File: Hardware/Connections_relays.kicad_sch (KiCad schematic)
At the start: 51 parts, among them J2 Conn_01x02, J3 1040310811, J4 Conn_01x02, J6 Conn_01x02, J7 Conn_01x02, Q11 IRLML0030, Q6 IRLML0030, Q8 IRLML0030, Q9 IRLML0030, U11 W25Q128JVS

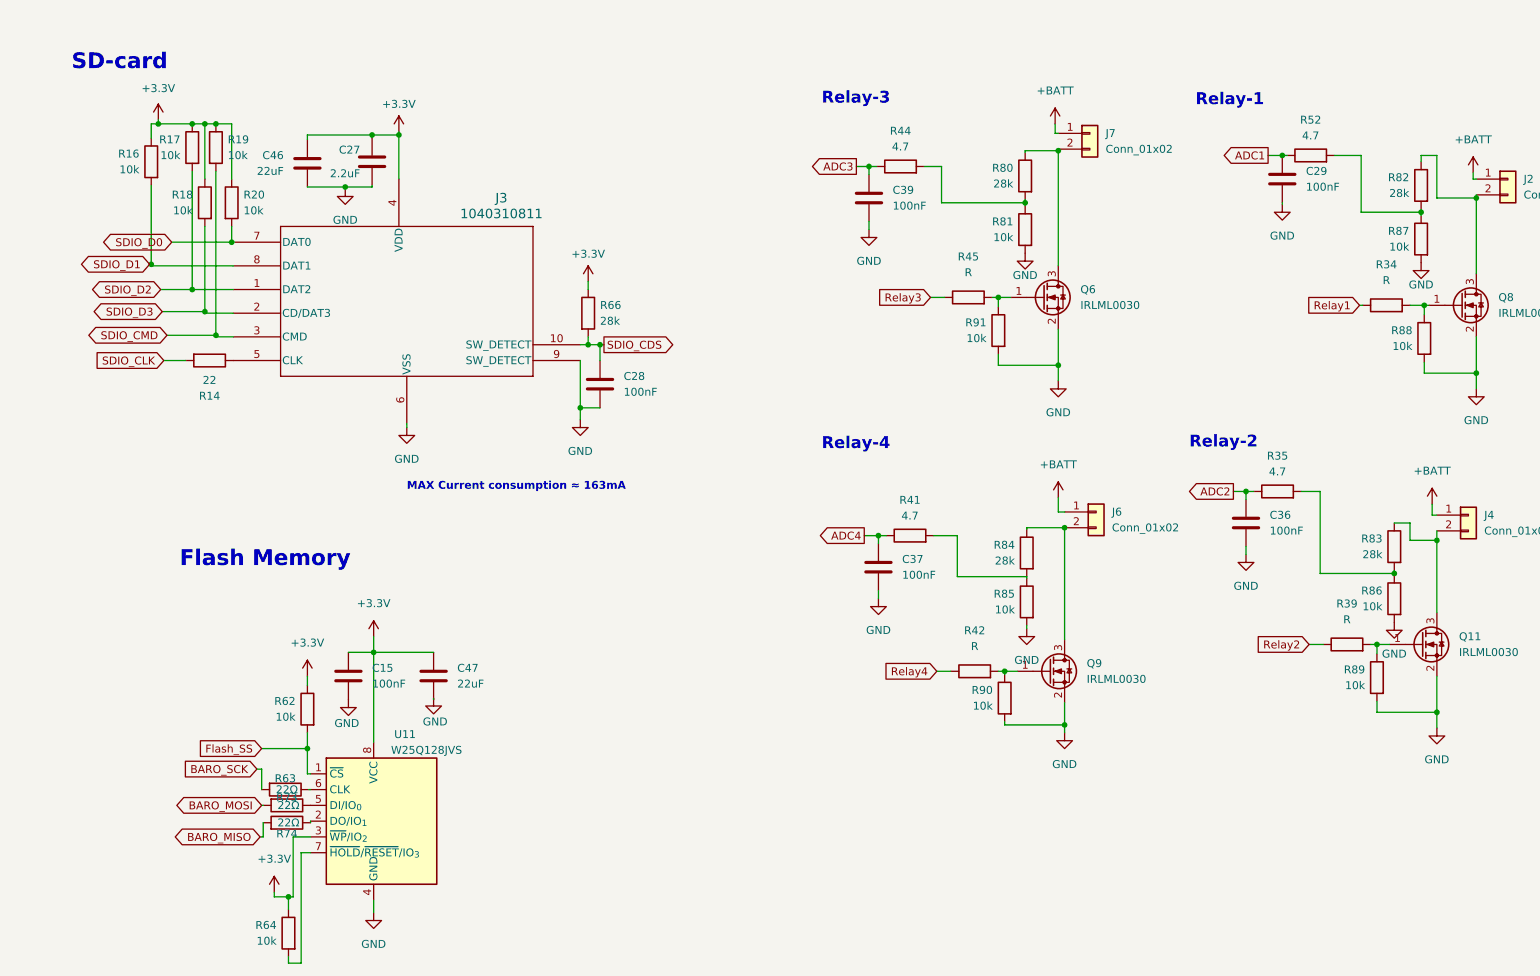
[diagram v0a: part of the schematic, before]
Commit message: Changed footprints, generated BOM
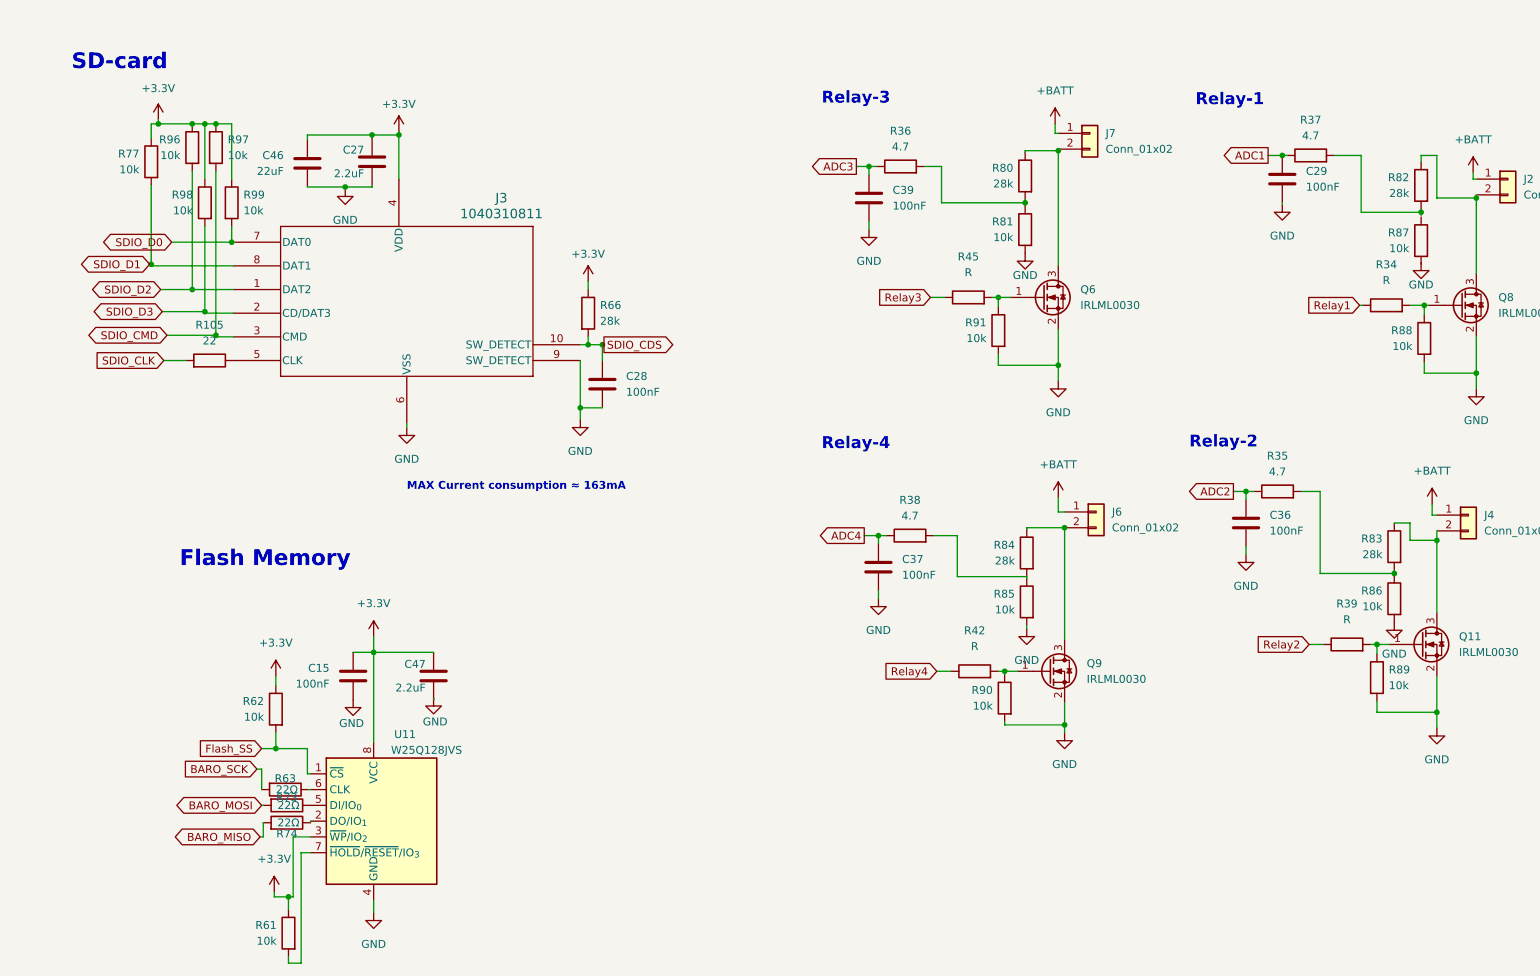
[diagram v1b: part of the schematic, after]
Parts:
- removed R14: 22, Resistor_SMD:R_0402_1005Metric, symbol Device:R
- removed R16, R17, R18, R19, R20, R64: 10k, Resistor_SMD:R_0402_1005Metric, symbol Device:R
- removed R41, R44, R52: 4.7, Resistor_SMD:R_0402_1005Metric, symbol Device:R
- added R105: 22, Resistor_SMD:R_0603_1608Metric, symbol Device:R
- added R36, R37, R38: 4.7, Resistor_SMD:R_0603_1608Metric, symbol Device:R
- added R61, R77, R96, R97, R98, R99: 10k, Resistor_SMD:R_0603_1608Metric, symbol Device:R
- C15, C28, C29, C36, C37, C39: footprint Capacitor_SMD:C_0402_1005Metric -> Capacitor_SMD:C_0603_1608Metric; Distributer Link https://www.ozdisan.com/p/smt-smd-ve-mlcc-kapasitorler-184/murata-grt155r71e104ke01d-1074547 -> https://www.ozdisan.com/p/smt-smd-ve-mlcc-kapasitorler-184/samsung-cl10b104ko8wpnc-522227; Part Number GRT155R71E104KE01D -> CL10B104KO8WPNC
- C27: footprint Capacitor_SMD:C_0402_1005Metric -> Capacitor_SMD:C_0603_1608Metric; Distributer Link http://ozdisan.com/p/smt-smd-ve-mlcc-kapasitorler-184/murat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 -> https://www.ozdisan.com/p/smt-smd-ve-mlcc-kapasitorler-184/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; Part Number GRT155C81A225ME13D -> CL10B225KP8NNNC
- C47: value 22uF -> 2.2uF; footprint Capacitor_SMD:C_0805_2012Metric -> Capacitor_SMD:C_0603_1608Metric; Distributer Link https://www.ozdisan.com/p/smt-smd-ve-mlcc-kapasitorler-184/samsung-cl21a226koqnnne-399002 -> https://www.ozdisan.com/p/smt-smd-ve-mlcc-kapasitorler-184/samsung-cl10b225kp8nnnc-359581; Part Number CL21A226KOQNNNE -> CL10B225KP8NNNC
- J2, J4, J6, J7: now left out of the parts list
- R35: footprint Resistor_SMD:R_0402_1005Metric -> Resistor_SMD:R_0603_1608Metric; Distributer Link https://www.ozdisan.com/p/smt-smd-ve-cip-direncler-194/royalohm-cq02wgj047jtce-587859 -> https://www.ozdisan.com/p/smt-smd-ve-cip-direncler-194/royalohm-cq03saf470kt5e-587940; Part Number CQ02WGJ047JTCE -> CQ03SAF470KT5E
- R62, R88, R89, R90, R91: footprint Resistor_SMD:R_0402_1005Metric -> Resistor_SMD:R_0603_1608Metric; Distributer Link https://www.ozdisan.com/p/smt-smd-ve-cip-direncler-194/roya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 -> https://www.ozdisan.com/p/smt-smd-ve-cip-direncler-194/viki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; Part Number CQ02WGF1002TCE -> CRT03J7E1002
- R81, R85, R86, R87: footprint Resistor_SMD:R_0402_1005Metric -> Resistor_SMD:R_0603_1608Metric; Distributer Link https://www.ozdisan.com/p/smt-smd-ve-cip-direncler-194/royalohm-cq02wgf1002tce-587902 -> https://www.ozdisan.com/p/smt-smd-ve-cip-direncler-194/royalohm-tc0350b1002t5f-700101; Part Number CQ02WGF1002TCE -> TC0350B1002T5F
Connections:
- net +3.3V: now also R61.1, R77.1, R96.1, R97.1, R98.1, R99.1
- net ADC1: now also R37.1
- net ADC3: now also R36.1
- net ADC4: now also R38.1
- net GND: no longer R87.2
- net SDIO_CLK: now also R105.2
- net SDIO_CMD: now also R97.2
- net SDIO_D0: now also R99.2
- net SDIO_D1: now also R77.2
- net SDIO_D2: now also R96.2
- net SDIO_D3: now also R98.2
- net at R80.2, R81.1: now also R36.2
- net at R82.2: now also R37.2; no longer R87.1
- net at J3.5 (CLK): now also R105.1
- net at R84.2, R85.1: now also R38.2
- net at U11.7 (~{HOLD}/~{RESET}/IO_{3}): now also R61.2

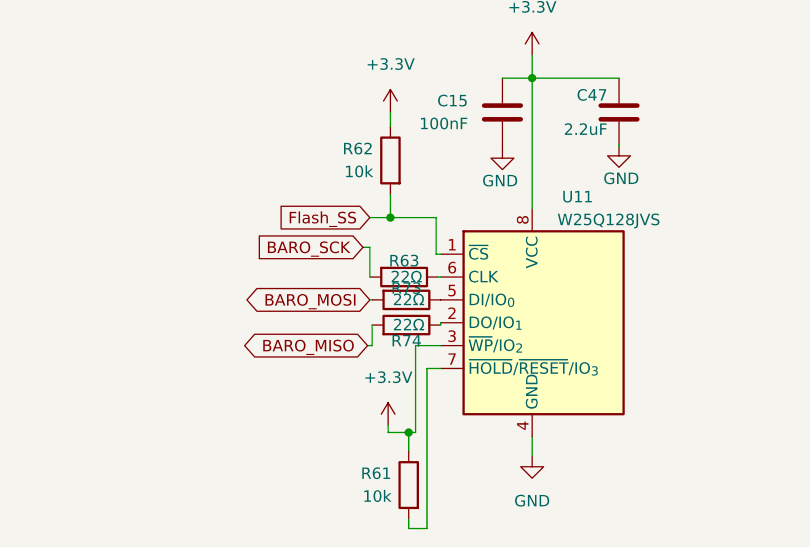
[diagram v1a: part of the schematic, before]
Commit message: Final changes
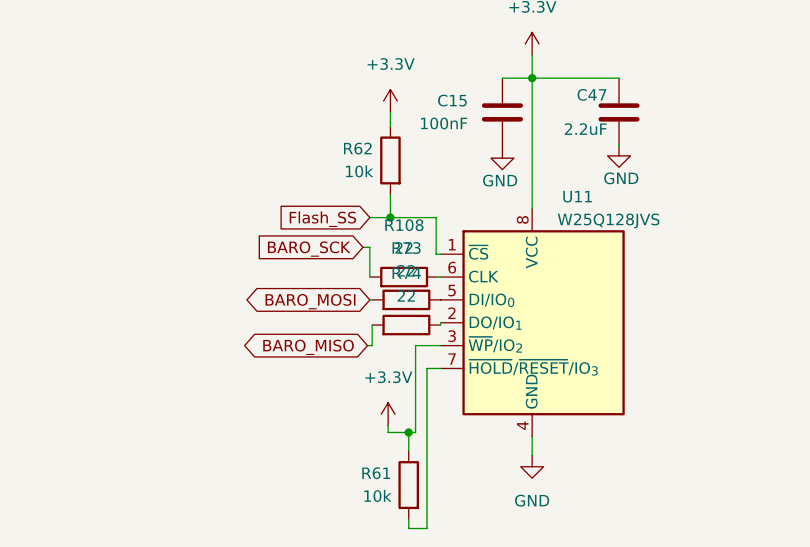
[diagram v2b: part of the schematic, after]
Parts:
- removed R63: 22Ω, Resistor_SMD:R_0402_1005Metric, symbol Device:R
- added R108: 22, Resistor_SMD:R_0603_1608Metric, symbol Device:R
- R73, R74: value 22Ω -> 22; footprint Resistor_SMD:R_0402_1005Metric -> Resistor_SMD:R_0603_1608Metric; Distributer Link https://www.ozdisan.com/p/smt-smd-ve-cip-direncler-194/pana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 -> https://www.ozdisan.com/p/smt-smd-ve-cip-direncler-194/roya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; Part Number ERJ2RKF22R0X -> CQ03SAJ0220T5E
- U11: Distributer Link https://www.ozdisan.com/en/p/embedded-memories-255/winbond-w25q32rvssjq-1580359?https://www.ozdisan.com/?utm_source=google&utm_medium=cpc&utm_campaign=creamake_pmax_en&utm_id=pmax-en&utm_term=%7Bkeyword%7D&utm_content=%7Bcreative%7D&gad_source=1&gad_campaignid=23758541728&gbraid=0AAAAADZaco-i9M5R6brnkfVhGNlfT6Ale&gclid=CjwKCAjw1IHTBhAaEiwA4AYNFgRblH-C799E_ndVsOY2spQbJEYXRXQi4HYBZksWK32CZ7DiI7YqRhoC9D4QAvD_BwE -> https://www.ozdisan.com/en/p/embedded-memories-255/winbond-w25q128jvsiq-525521; Part Number W25Q32RVSSJQ -> W25Q128JVSIQ
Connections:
- net BARO_SCK: now also R108.2
- net at U11.6 (CLK): now also R108.1
